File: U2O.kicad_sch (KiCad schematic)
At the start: 21 parts, among them J1 AFBR-1624Z, J2 USB_B_Micro, J3 AFBR-2624Z, U1 CP2102N-Axx-xQFN20

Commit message: one more time
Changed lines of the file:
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@@
 (kicad_sch
-	(version 20231120)
+	(version 20250114)
 	(generator "eeschema")
-	(generator_version "8.0")
+	(generator_version "9.0")
 	(paper "A4")
+	(rectangle
+		(start 110.49 16.51)
+		(end 177.8 68.58)
+		(stroke
+			(width 0)
+			(type default)
+		)
+		(fill
+			(type none)
+		)
+	)
+	(rectangle
+		(start 64.77 97.79)
+		(end 87.63 128.27)
+		(stroke
+			(width 0)
+			(type default)
+		)
+		(fill
+			(type none)
+		)
+	)
+	(rectangle
+		(start 110.49 73.66)
+		(end 177.8 125.73)
+		(stroke
+			(width 0)
+			(type default)
+		)
+		(fill
+			(type none)
+		)
+	)
+	(rectangle
+		(start 16.51 16.51)
+		(end 48.26 52.07)
+		(stroke
+			(width 0)
+			(type default)
+		)
+		(fill
+			(type none)
+		)
+	)
+	(rectangle
+		(start 16.51 97.79)
+		(end 39.37 128.27)
+		(stroke
+			(width 0)
+			(type default)
+		)
+		(fill
+			(type none)
+		)
+	)
+	(rectangle
+		(start 16.51 57.15)
+		(end 48.26 92.71)
+		(stroke
+			(width 0)
+			(type default)
+		)
+		(fill
+			(type none)
+		)
+	)
+	(rectangle
+		(start 49.53 16.51)
+		(end 109.22 92.71)
+		(stroke
+			(width 0)
+			(type default)
+		)
+		(fill
+			(type none)
+		)
+	)
+	(rectangle
+		(start 40.64 97.79)
+		(end 63.5 128.27)
+		(stroke
+			(width 0)
+			(type default)
+		)
+		(fill
+			(type none)
+		)
+	)
+	(text "Serial Converter (UART)"
+		(exclude_from_sim no)
+		(at 79.502 95.504 0)
+		(effects
+			(font
+				(size 1.27 1.27)
+			)
+		)
+	)
+	(text "Voltage Divider\n"
+		(exclude_from_sim no)
+		(at 32.004 94.996 0)
+		(effects
+			(font
+				(size 1.27 1.27)
+			)
+		)
+	)
+	(text "Ripple Protection"
+		(exclude_from_sim no)
+		(at 28.194 130.556 0)
+		(effects
+			(font
+				(size 1.27 1.27)
+			)
+		)
+	)
+	(text "USB Connection\n"
+		(exclude_from_sim no)
+		(at 32.004 54.102 0)
+		(effects
+			(font
+				(size 1.27 1.27)
+			)
+		)
+	)
+	(text "Transmitter\n"
+		(exclude_from_sim no)
+		(at 143.764 71.12 0)
+		(effects
+			(font
+				(size 1.27 1.27)
+			)
+		)
+	)
+	(text "ESD Protection"
+		(exclude_from_sim no)
+		(at 75.946 130.302 0)
+		(effects
+			(font
+				(size 1.27 1.27)
+			)
+		)
+	)
+	(text "Ripple Protection"
+		(exclude_from_sim no)
+		(at 52.07 130.556 0)
+		(effects
+			(font
+				(size 1.27 1.27)
+			)
+		)
+	)
+	(text "Receiver"
+		(exclude_from_sim no)
+		(at 144.78 127.762 0)
+		(effects
+			(font
+				(size 1.27 1.27)
+			)
+		)
+	)
 	(junction
 		(at 156.21 25.4)
@@
 		)
 	)
-	(rectangle
-		(start 110.49 16.51)
-		(end 177.8 68.58)
-		(stroke
-			(width 0)
-			(type default)
-		)
-		(fill
-			(type none)
-		)
-	)
-	(rectangle
-		(start 64.77 97.79)
-		(end 87.63 128.27)
-		(stroke
-			(width 0)
-			(type default)
-		)
-		(fill
-			(type none)
-		)
-	)
-	(rectangle
-		(start 110.49 73.66)
-		(end 177.8 125.73)
-		(stroke
-			(width 0)
-			(type default)
-		)
-		(fill
-			(type none)
-		)
-	)
-	(rectangle
-		(start 16.51 16.51)
-		(end 48.26 52.07)
-		(stroke
-			(width 0)
-			(type default)
-		)
-		(fill
-			(type none)
-		)
-	)
-	(rectangle
-		(start 16.51 97.79)
-		(end 39.37 128.27)
-		(stroke
-			(width 0)
-			(type default)
-		)
-		(fill
-			(type none)
-		)
-	)
-	(rectangle
-		(start 16.51 57.15)
-		(end 48.26 92.71)
-		(stroke
-			(width 0)
-			(type default)
-		)
-		(fill
-			(type none)
-		)
-	)
-	(rectangle
-		(start 49.53 16.51)
-		(end 109.22 92.71)
-		(stroke
-			(width 0)
-			(type default)
-		)
-		(fill
-			(type none)
-		)
-	)
-	(rectangle
-		(start 40.64 97.79)
-		(end 63.5 128.27)
-		(stroke
-			(width 0)
-			(type default)
-		)
-		(fill
-			(type none)
-		)
-	)
-	(text "Serial Converter (UART)"
-		(exclude_from_sim no)
-		(at 79.502 95.504 0)
-		(effects
-			(font
-				(size 1.27 1.27)
-			)
-		)
-	)
-	(text "Voltage Divider\n"
-		(exclude_from_sim no)
-		(at 32.004 94.996 0)
-		(effects
-			(font
-				(size 1.27 1.27)
-			)
-		)
-	)
-	(text "Ripple Protection"
-		(exclude_from_sim no)
-		(at 28.194 130.556 0)
-		(effects
-			(font
-				(size 1.27 1.27)
-			)
-		)
-	)
-	(text "USB Connection\n"
-		(exclude_from_sim no)
-		(at 32.004 54.102 0)
-		(effects
-			(font
-				(size 1.27 1.27)
-			)
-		)
-	)
-	(text "Transmitter\n"
-		(exclude_from_sim no)
-		(at 143.764 71.12 0)
-		(effects
-			(font
-				(size 1.27 1.27)
-			)
-		)
-	)
-	(text "ESD Protection"
-		(exclude_from_sim no)
-		(at 75.946 130.302 0)
-		(effects
-			(font
-				(size 1.27 1.27)
-			)
-		)
-	)
-	(text "Ripple Protection"
-		(exclude_from_sim no)
-		(at 52.07 130.556 0)
-		(effects
-			(font
-				(size 1.27 1.27)
-			)
-		)
-	)
-	(text "Receiver"
-		(exclude_from_sim no)
-		(at 144.78 127.762 0)
-		(effects
-			(font
-				(size 1.27 1.27)
-			)
-		)
-	)
 	(global_label "D-"
 		(shape input)
@@
 		)
 	)
+	(embedded_fonts no)
 )

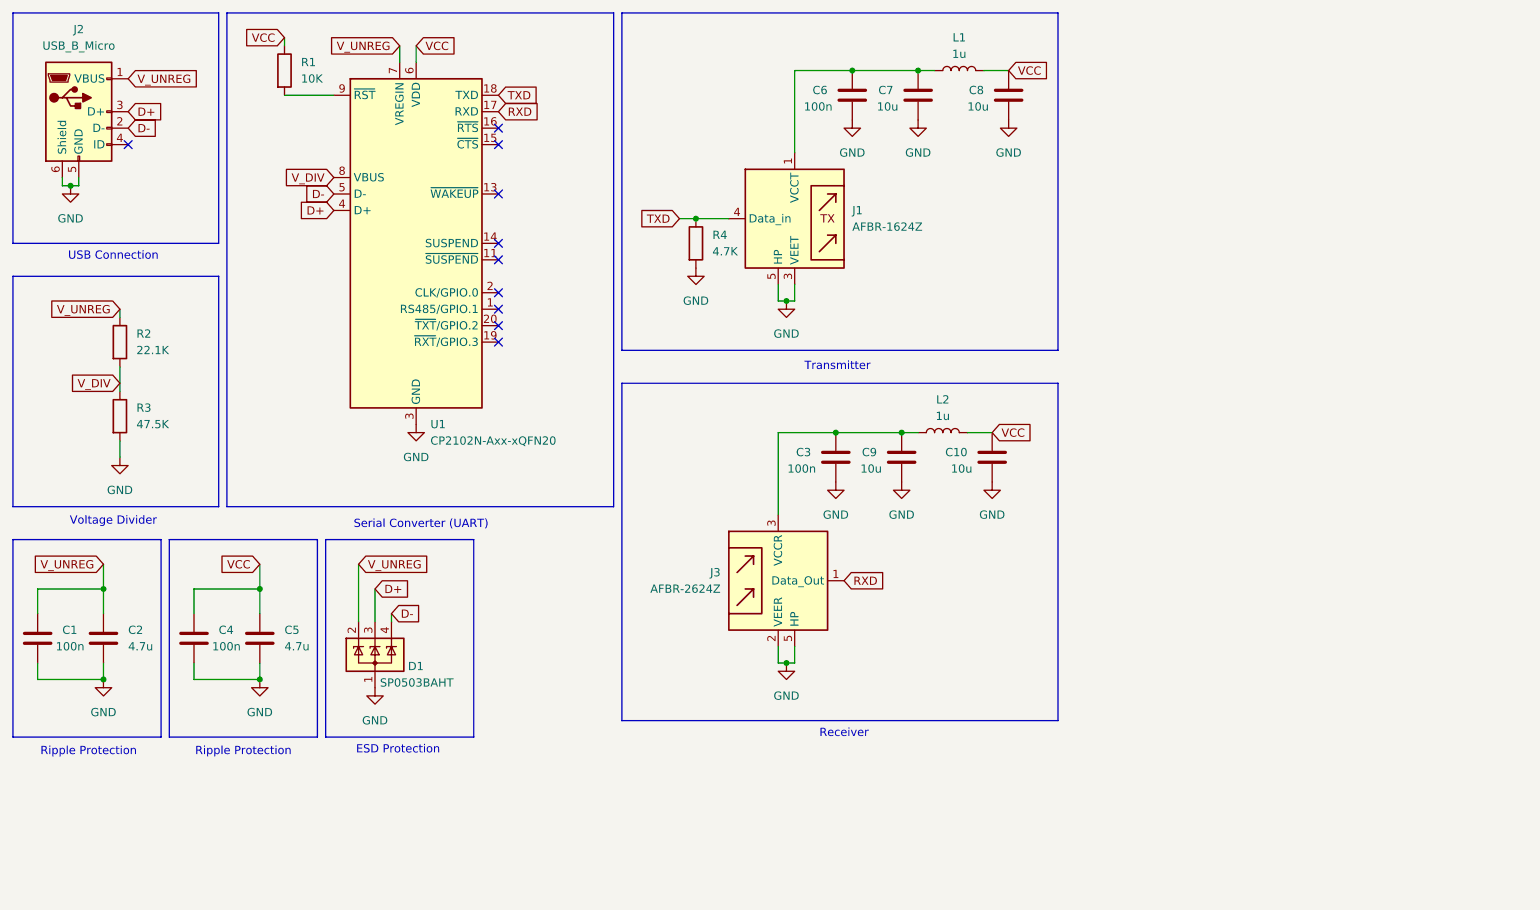
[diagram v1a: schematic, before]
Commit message: final push
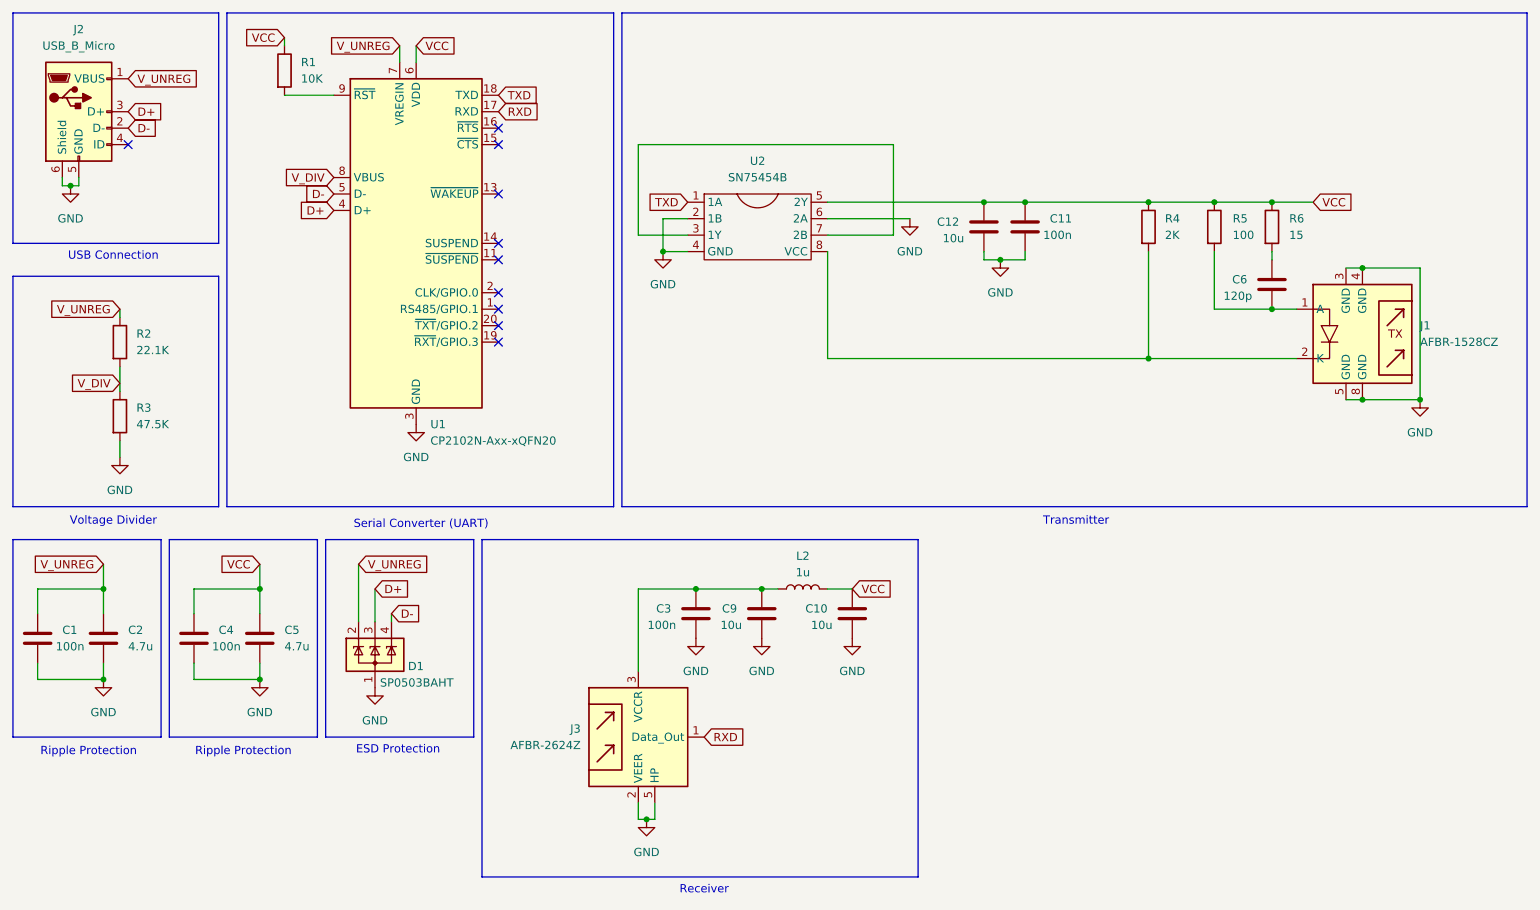
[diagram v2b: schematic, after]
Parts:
- removed C7, C8: 10u, Capacitor_SMD:C_0603_1608Metric, symbol Device:C
- removed L1: 1u, Inductor_SMD:L_0603_1608Metric, symbol Device:L
- added C11: 100n, Capacitor_SMD:C_0603_1608Metric, symbol Device:C
- added C12: 10u, Capacitor_SMD:C_0603_1608Metric, symbol Device:C
- added R5: 100, Resistor_SMD:R_0603_1608Metric, symbol Device:R
- added R6: 15, Resistor_SMD:R_0603_1608Metric, symbol Device:R
- added U2: SN75454B, Package_DIP:DIP-8_W7.62mm, symbol mannual Components:SN75454B
- C6: value 100n -> 120p
- J1: value AFBR-1624Z -> AFBR-1528CZ
- R4: value 4.7K -> 2K
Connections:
- net GND: now also J1.4 (GND), C11.2, C12.1, U2.2 (1B), U2.4 (GND), U2.6 (2A); no longer C6.1, R4.2
- net TXD: now also U2.1 (1A); no longer J1.4 (Data_in), R4.1
- net VCC: now also R4.1, C11.1, C12.2, R5.1, R6.1, U2.5 (2Y)
- net at J1.1 (A): now also C6.1, R5.2; no longer C6.2
- new net: C6.2, R6.2
- new net: U2.3 (1Y), U2.7 (2B)
- new net: J1.2 (NC), R4.2, U2.8 (VCC)
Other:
- moved on the sheet: C10, C3, C6, C9, J3, L2, R4
